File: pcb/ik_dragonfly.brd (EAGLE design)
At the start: 41.1 x 20.3 mm, 32 parts, among them IC1 ATXMEGA32E5, IC2 FT230X, J1 2X03, U1 MIC5219-3.3, U2 LM4040

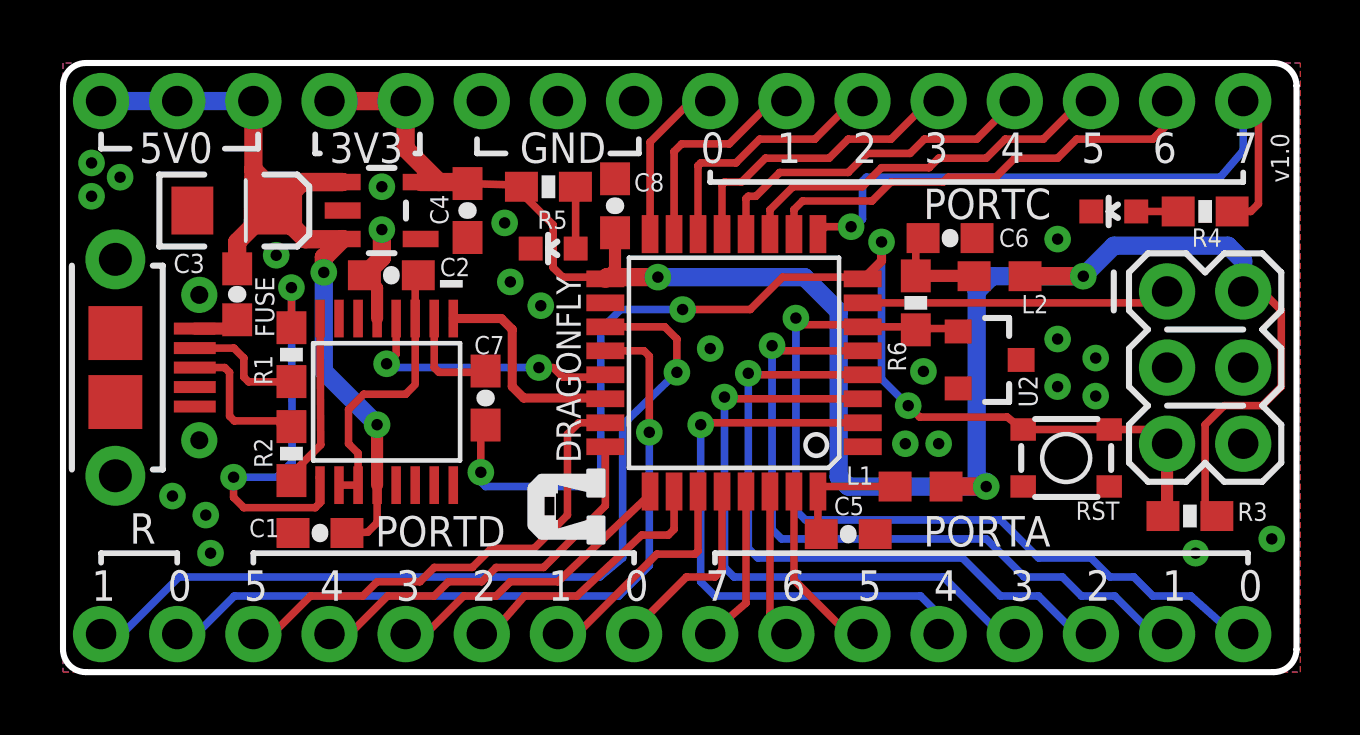
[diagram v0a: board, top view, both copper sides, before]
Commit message: finished (for reals) BOM
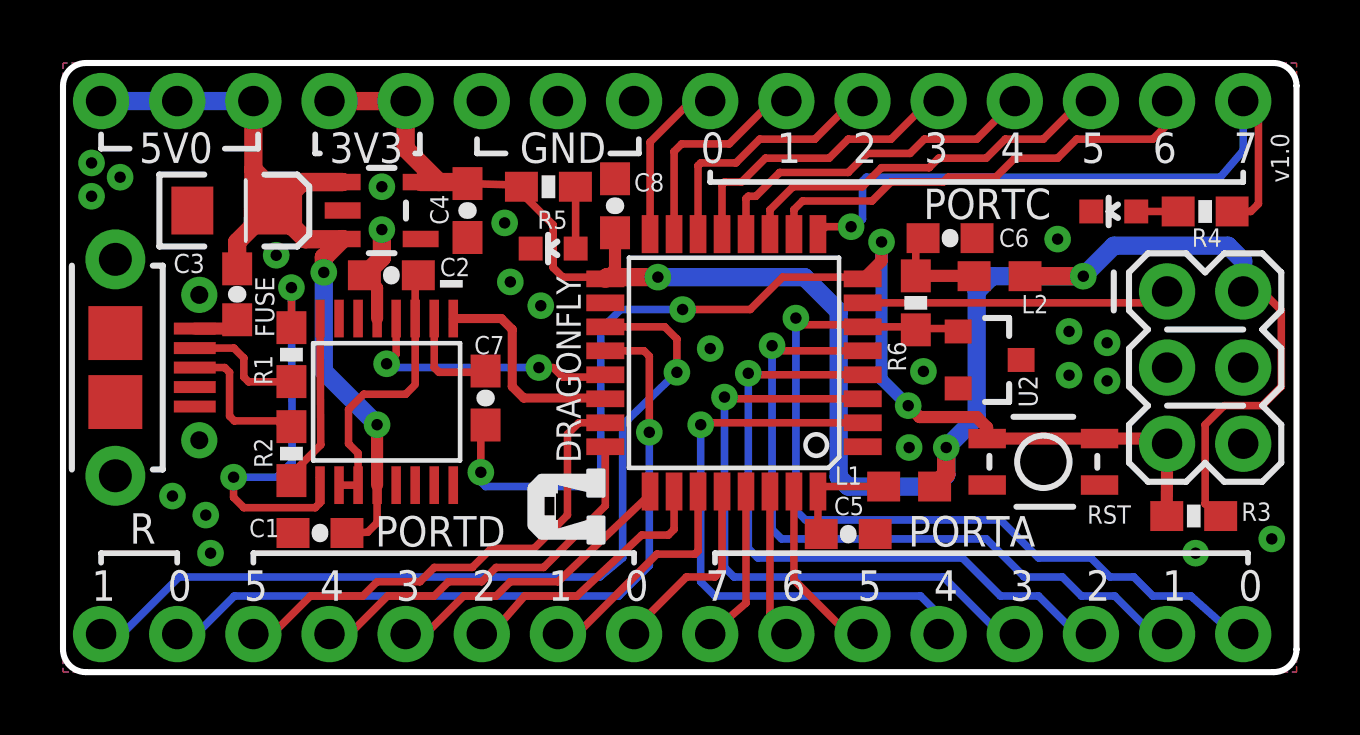
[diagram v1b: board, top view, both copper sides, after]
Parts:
- RST: device Ai_Electromechanical:SW-SPST-SMD03X026 -> Ai_Electromechanical:SW-SPST-SMD035X030
- moved RST 0.77 mm to (32.7, 7.02)
- moved L1 0.38 mm to (28.2, 6.19)
- moved R3 0.13 mm to (37.7, 5.21)
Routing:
- net 3V3: track 66.4 -> 64.9 mm
- net GND: vias 23 -> 22

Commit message: minor revision
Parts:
- LOGO1: device SparkFun-Aesthetics:OSHW-LOGO-S -> Ai_Miscellany:OSHW-LOGO-S
- RST: value SW-SPSTSMD03X026 -> SW-SPSTSMD035X030
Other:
- board text added: "By Ihsan Kehribar"
- board text removed: "Ihsan Kehribar"
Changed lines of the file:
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@@
 <setting verticaltext="up"/>
 </settings>
-<grid distance="5" unitdist="mil" unit="mil" style="lines" multiple="1" display="yes" altdistance="0.025" altunitdist="inch" altunit="inch"/>
+<grid distance="0.05" unitdist="inch" unit="inch" style="lines" multiple="1" display="yes" altdistance="0.025" altunitdist="inch" altunit="inch"/>
 <layers>
 <layer number="1" name="Top" color="4" fill="1" visible="yes" active="yes"/>
@@
 <wire x1="11.90625" y1="17.93875" x2="11.90625" y2="17.30375" width="0.1905" layer="21"/>
 <wire x1="11.7475" y1="17.30375" x2="11.90625" y2="17.30375" width="0.1905" layer="21"/>
-<text x="29.4005" y="15.60195" size="1.524" layer="22" ratio="15" rot="MR0">ATxmega32E5</text>
 <dimension x1="41.148" y1="20.32" x2="0" y2="20.32" x3="20.574" y3="22.06625" textsize="1.778" textratio="15" layer="49"/>
-<text x="15.367" y="7.20725" size="1.016" layer="22" font="vector" ratio="15" rot="MR180">Ihsan Kehribar</text>
-<text x="14.224" y="5.55625" size="1.016" layer="22" font="vector" ratio="15" rot="MR180">www.acrobotic.com</text>
+<text x="16.129" y="6.44525" size="0.8128" layer="22" font="vector" ratio="15" rot="MR180">By Ihsan Kehribar</text>
+<text x="16.51" y="5.04825" size="0.8128" layer="22" font="vector" ratio="15" rot="MR180">www.acrobotic.com</text>
 <text x="40.90035" y="16.3322" size="0.6096" layer="21" font="vector" ratio="15" rot="R90">v1.0</text>
 <text x="17.272" y="6.985" size="0.8128" layer="21" font="vector" ratio="15" rot="R90">DRAGONFLY</text>
+<text x="27.8765" y="16.61795" size="1.27" layer="22" ratio="15" rot="MR0">DRAGONFLY</text>
+<text x="26.6065" y="15.34795" size="0.8128" layer="22" ratio="15" rot="MR0">ATxmega32E5</text>
 </plain>
 <attributes>
@@
 </element>
 <element name="ON" library="Ai_LED" package="LED-0603" value="BLUE" x="16.35125" y="14.12875" smashed="yes" rot="R90"/>
-<element name="LOGO1" library="SparkFun-Aesthetics" package="OSHW-LOGO-S" value="OSHW-LOGOS" x="22.352" y="13.208" smashed="yes" rot="MR0"/>
+<element name="LOGO1" library="Ai_Miscellany" package="OSHW-LOGO-S" value="OSHW-LOGOS" x="22.352" y="13.208" smashed="yes" rot="MR0"/>
 <element name="R6" library="Ai_Passives" package="RES-0603" value="1K" x="28.448" y="12.319" smashed="yes" rot="R90">
 <attribute name="NAME" x="28.12415" y="10.02665" size="0.6096" layer="25" font="vector" ratio="15" rot="R90"/>
@@
 </element>
 <element name="USB1" library="Ai_Connectors" package="USB-MICROB-TH" value="USBMICROB-TH" x="1.74625" y="10.16" smashed="yes" rot="R270"/>
-<element name="RST" library="Ai_Electromechanical" package="SW-SPST-SMD035X030" value="SW-SPSTSMD03X026" x="32.7025" y="7.01675" smashed="yes" rot="R180">
+<element name="RST" library="Ai_Electromechanical" package="SW-SPST-SMD035X030" value="SW-SPSTSMD035X030" x="32.7025" y="7.01675" smashed="yes" rot="R180">
 <attribute name="NAME" x="34.163" y="4.953" size="0.6096" layer="21" font="vector" ratio="15"/>
 </element>
